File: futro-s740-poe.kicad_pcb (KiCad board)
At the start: 2 copper layers, 66 x 37 mm, 9 parts, among them J1 Conn_02x08, J2 Conn_02x08, U1 SM51589PEL, U2 AG5412

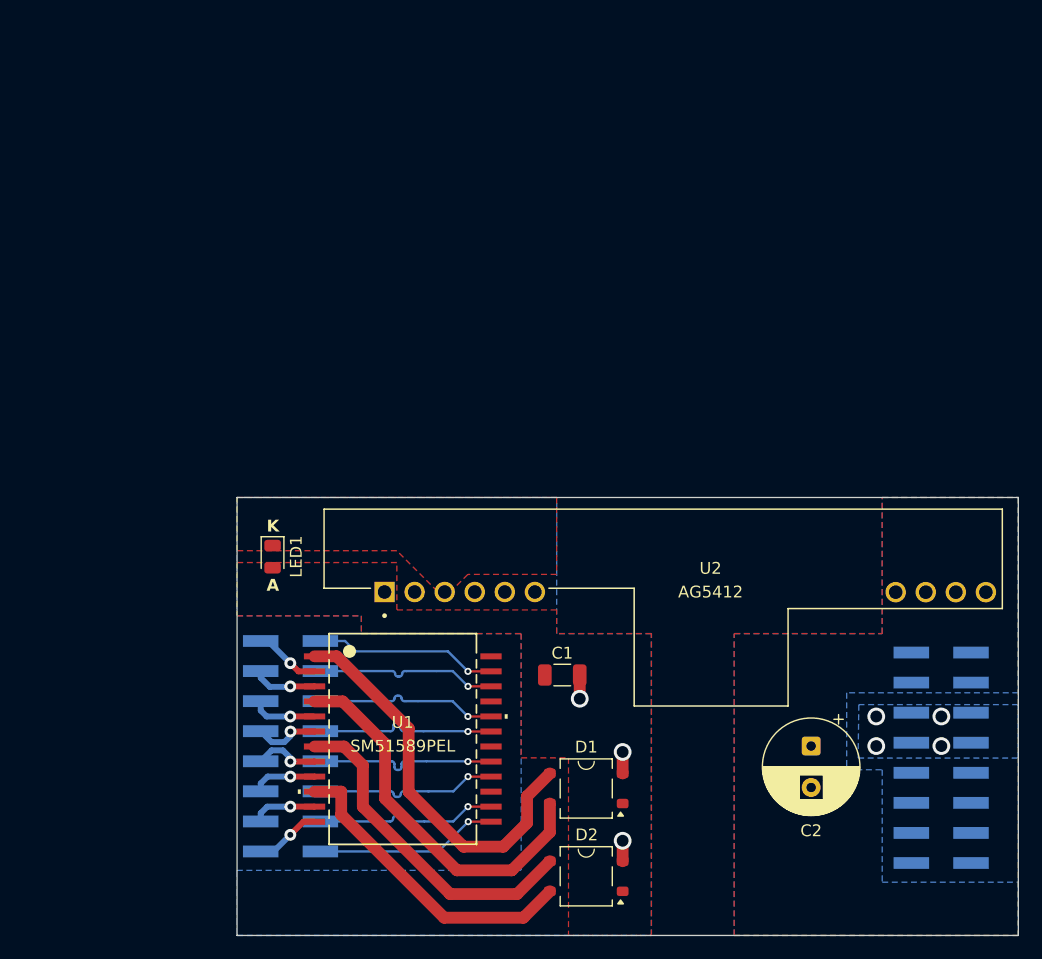
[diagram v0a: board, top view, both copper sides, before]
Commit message: migrated to new structure
Signed-off-by: Takuto Nagami <logica0419@gmail.com>
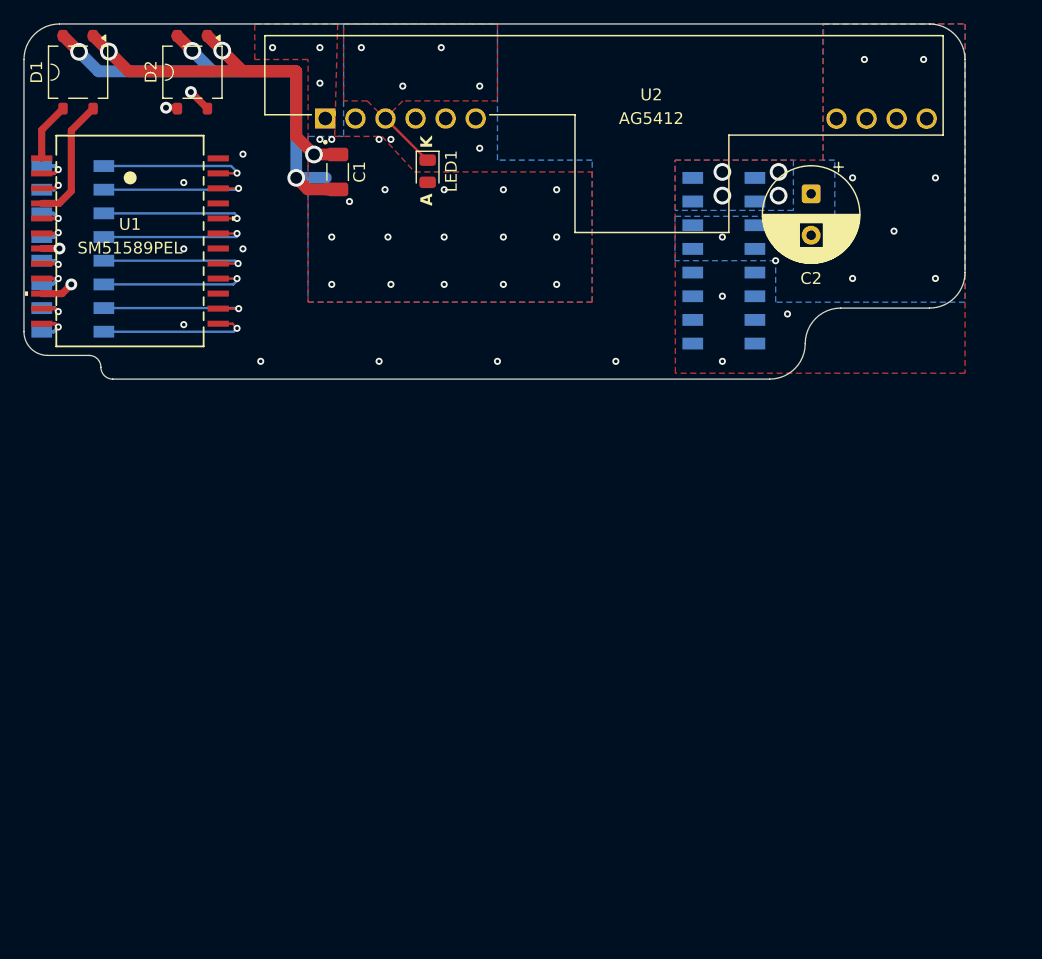
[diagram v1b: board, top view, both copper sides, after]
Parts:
- J1, J2: footprint Connector_PinSocket_2.54mm:PinSocket_2x08_P2.54mm_Vertical_SMD -> Connector_PinSocket_2.00mm:PinSocket_2x08_P2.00mm_Vertical_SMD
- moved D2 75.6 mm to (34.2, 22.1), turned to -90 degrees
- moved D1 74.2 mm to (24.6, 22.1), turned to -90 degrees
- moved U1 48.0 mm to (29.0, 36.3)
- moved C2 46.7 mm to (86.5, 32.3)
- moved C1 46.5 mm to (46.5, 30.5), turned to -90 degrees
- moved J1 45.9 mm to (24.1, 37.0)
- moved J2 45.8 mm to (79.1, 38.0)
- moved U2 40.3 mm to (69.0, 26.0)
- moved LED1 35.1 mm to (54.1, 30.4)
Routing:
- net Net-(D1--): track 5.54 -> 74.6 mm, vias 3 -> 18
- net Net-(D1-+): track 0.00 -> 63.4 mm, vias 0 -> 15
- net Net-(U1-MCT1): track 33.6 -> 4.95 mm
- net Net-(U1-MCT2): track 32.3 -> 10.7 mm
- net Net-(U1-MCT3): track 28.2 -> 21.7 mm, vias 0 -> 2
- net Net-(LED1-K): track 0.00 -> 5.05 mm
- net Net-(U1-MCT4): track 26.4 -> 29.3 mm, vias 0 -> 2
- net Net-(J1-Pin_1): track 5.61 -> 3.06 mm
- net Net-(J1-Pin_9): track 5.50 -> 2.96 mm
- net Net-(J1-Pin_7): track 5.52 -> 2.98 mm
- net Net-(J1-Pin_5): track 5.51 -> 2.98 mm
- net Net-(J1-Pin_15): track 5.59 -> 3.08 mm
- net Net-(J1-Pin_11): track 5.45 -> 3.00 mm
- net Net-(J1-Pin_13): track 5.47 -> 3.03 mm
- net Net-(J1-Pin_3): track 5.45 -> 3.06 mm
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- added copper zone on In1.Cu, net Net-(D1-+)
- added copper zone on In2.Cu, net Net-(D1--)
- added copper zone on F.Cu, net Net-(J2-Pin_1)
- added copper zone on In1.Cu, net Net-(J2-Pin_5)
- added copper zone on In2.Cu, net Net-(J2-Pin_5)
- removed copper zone on F.Cu, net Net-(J2-Pin_5)
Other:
- board size 66 x 37 mm -> 79.5 x 30 mm
- copper layers 2 -> 4
